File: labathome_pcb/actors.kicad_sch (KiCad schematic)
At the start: 33 parts, among them J26 Servos, J7 FAN5V, J8 3V GN RGB 5V, Q1 BC817, Q2 IRLML6344, Q3 MJD31C, Q5 IRLML6344, X1 FAN_6024

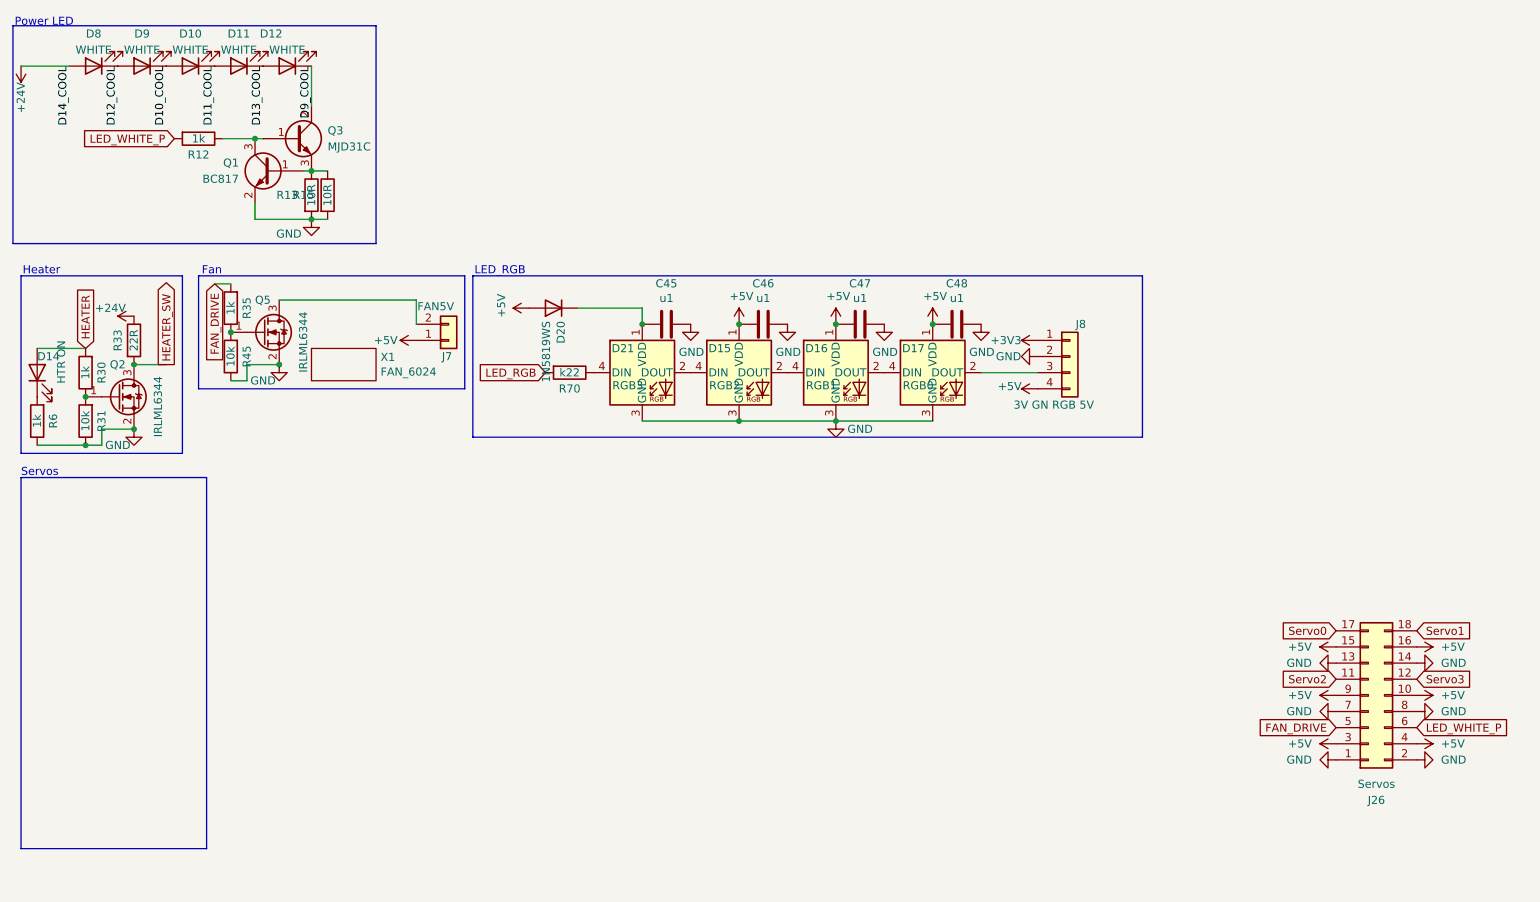
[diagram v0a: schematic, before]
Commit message: Optimized PCB
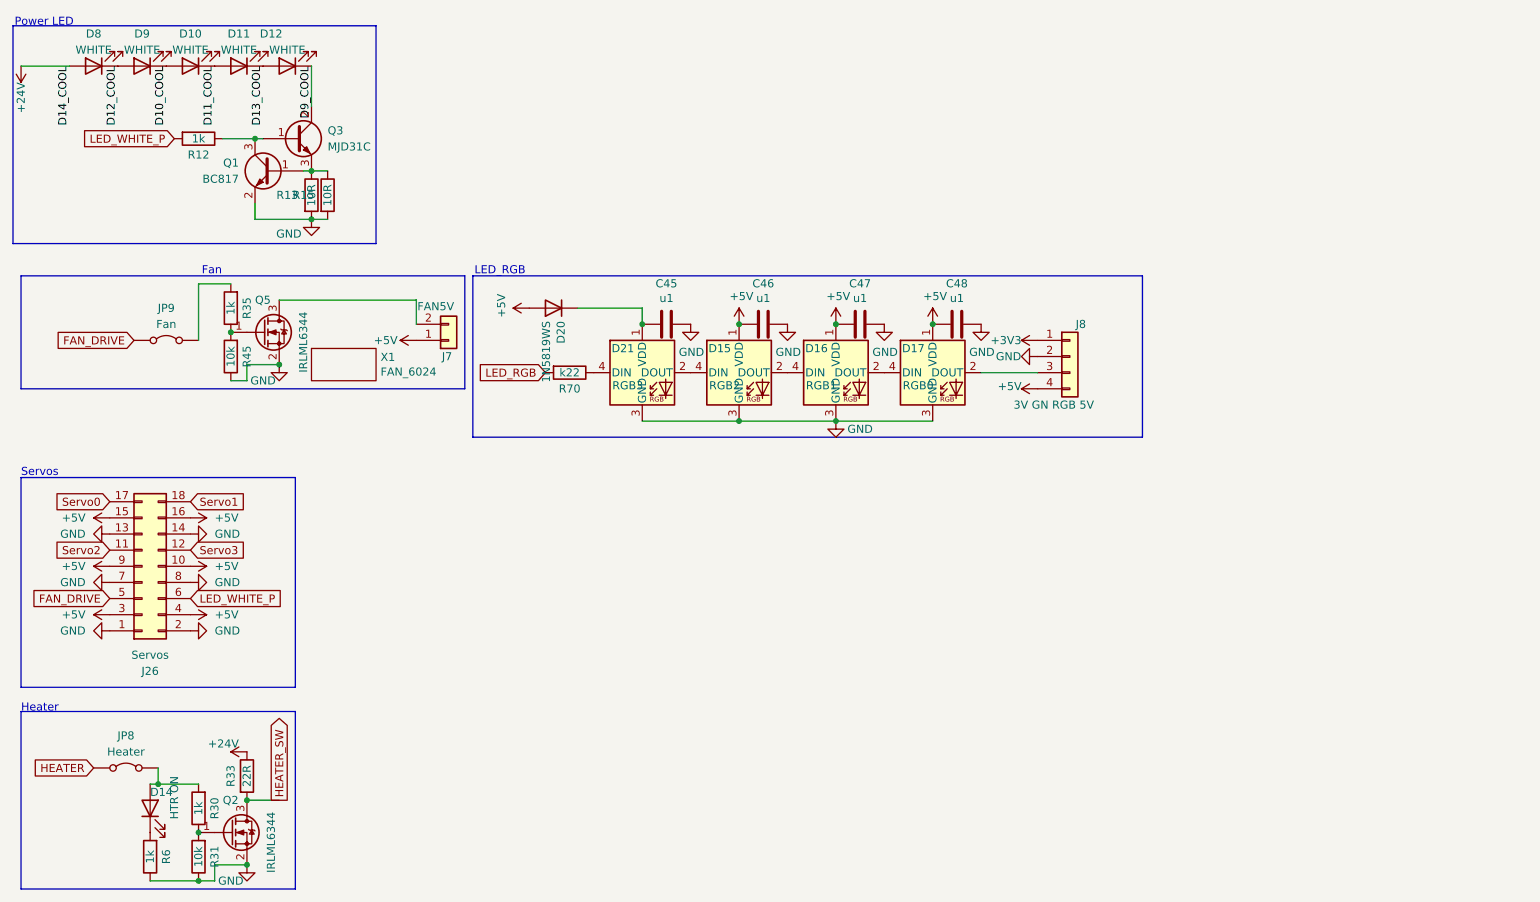
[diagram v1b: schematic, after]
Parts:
- added JP8: Heater, Jumper:SolderJumper-2_P1.3mm_Bridged2Bar_RoundedPad1.0x1.5mm, symbol Jumper:Jumper_2_Bridged
- added JP9: Fan, Jumper:SolderJumper-2_P1.3mm_Bridged2Bar_RoundedPad1.0x1.5mm, symbol Jumper:Jumper_2_Bridged
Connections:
- net FAN_DRIVE: now also JP9.1 (A); no longer R35.2
- net HEATER: now also JP8.1 (A); no longer D14.2 (A), R30.2
- new net: D14.2 (A), JP8.2 (B), R30.2
- new net: JP9.2 (B), R35.2
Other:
- moved on the sheet: D14, J26, Q2, R30, R31, R33, R6
